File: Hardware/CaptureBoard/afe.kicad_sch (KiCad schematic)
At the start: 64 parts, among them J801 Conn_02x05_Odd_Even, U800 AD9978, U801 ICE40HX4K-BG121, U802 W25Q32JVZP, U803 ADA4800, U804 ADA4800, X801 33.33MHz

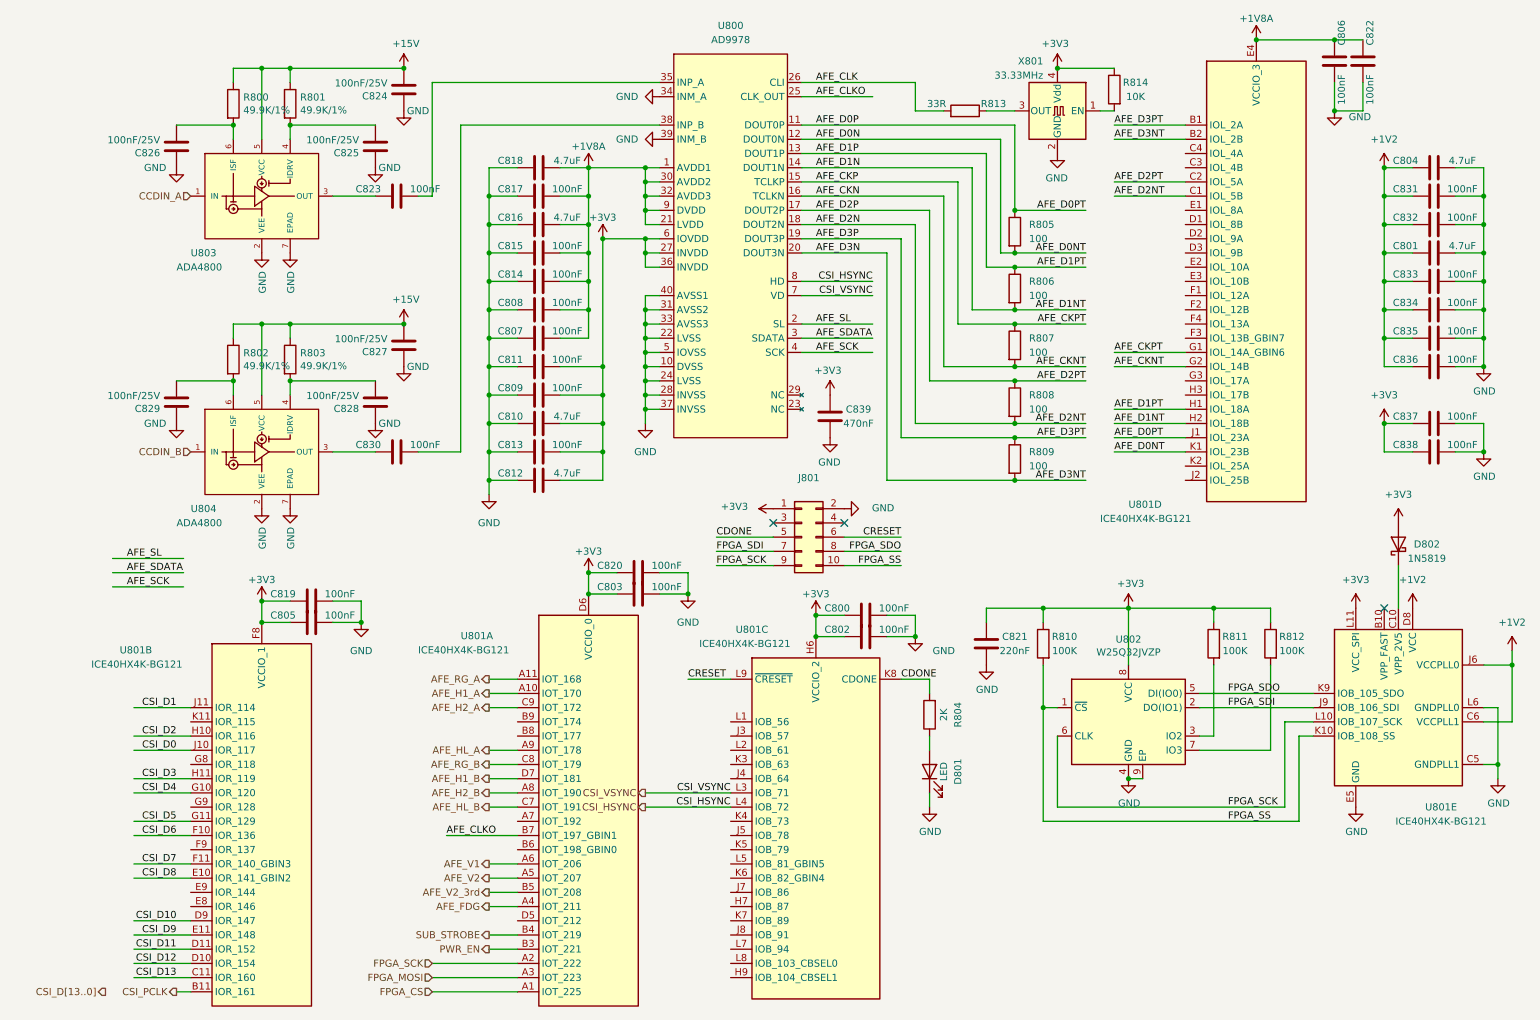
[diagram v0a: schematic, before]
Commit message: pcb: PB r0p2 and CB r0p3 freeze
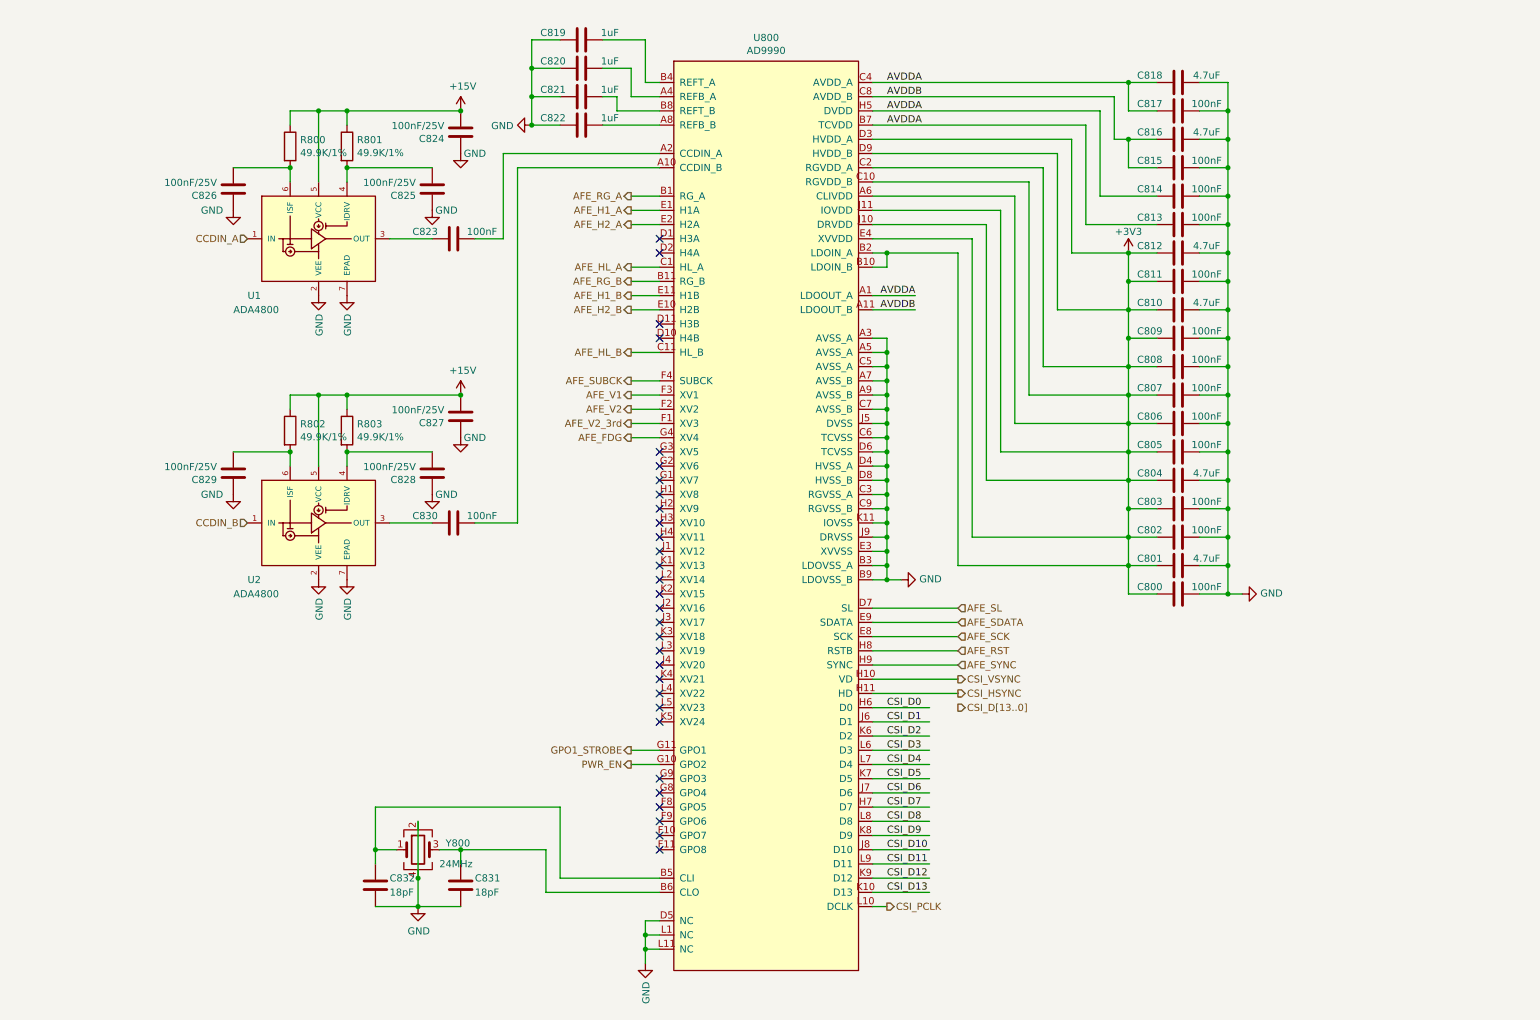
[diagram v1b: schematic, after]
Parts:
- removed C833, C834, C835, C836, C837, C838: 100nF, Capacitor_SMD:C_0402_1005Metric, symbol Device:C
- removed C839: 470nF, Capacitor_SMD:C_0402_1005Metric, symbol Device:C
- removed D801: LED, Diode_SMD:D_0603_1608Metric, symbol Device:LED
- removed D802: 1N5819, Diode_SMD:D_SOD-123, symbol Diode:MBR0530
- removed J801: Conn_02x05_Odd_Even, Connector_PinHeader_1.27mm:PinHeader_2x05_P1.27mm_Vertical_SMD, symbol Connector_Generic:Conn_02x05_Odd_Even
- removed R804: 2K, Resistor_SMD:R_0402_1005Metric, symbol Device:R
- removed R805, R806, R807, R808, R809: 100, Resistor_SMD:R_0402_1005Metric, symbol Device:R
- removed R810, R811, R812: 100K, Resistor_SMD:R_0402_1005Metric, symbol Device:R
- removed R813: 33R, Capacitor_SMD:C_0402_1005Metric, symbol Device:R
- removed R814: 10K, Capacitor_SMD:C_0402_1005Metric, symbol Device:R
- removed U800: AD9978, Package_DFN_QFN:QFN-40-1EP_6x6mm_P0.5mm_EP4.6x4.6mm, symbol Sitina:AD9978
- removed U801: ICE40HX4K-BG121, Package_BGA:BGA-121_9.0x9.0mm_Layout11x11_P0.8mm_Ball0.4mm_Pad0.35mm_NSMD, symbol FPGA_Lattice:ICE40HX4K-BG121
- removed U802: W25Q32JVZP, Package_SON:WSON-8-1EP_6x5mm_P1.27mm_EP3.4x4.3mm, symbol Memory_Flash:W25Q32JVZP
- removed X801: 33.33MHz, Oscillator:Oscillator_SMD_Abracon_ASE-4Pin_3.2x2.5mm, symbol Oscillator:ASE-xxxMHz
- added U800: AD9990, Footprints:BGA-112_11x11_8.0x8.0mm, symbol Sitina:AD9990
- added Y800: 24MHz, Crystal:Crystal_SMD_3225-4Pin_3.2x2.5mm, symbol Device:Crystal_GND24
- C819, C820, C822: value 100nF -> 1uF
- C821: value 220nF -> 1uF
- C831, C832: value 100nF -> 18pF; footprint Capacitor_SMD:C_0402_1005Metric -> Capacitor_SMD:C_0603_1608Metric
- U1: renamed from U803; footprint Package_DFN_QFN:DFN-6-1EP_2x2mm_P0.5mm_EP0.6x1.37mm -> Package_DFN_QFN:DFN-6-1EP_2x1.8mm_P0.5mm_EP1.2x1.6mm
- U2: renamed from U804; footprint Package_DFN_QFN:DFN-6-1EP_2x2mm_P0.5mm_EP0.6x1.37mm -> Package_DFN_QFN:DFN-6-1EP_2x1.8mm_P0.5mm_EP1.2x1.6mm
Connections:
- net +3V3: now also C801.2, C804.2, C806.2, C807.2, C808.2, C809.2, C810.2, C811.2, C812.2, U800.A6 (CLIVDD), U800.B10 (LDOIN_B), U800.B2 (LDOIN_A), U800.C10 (RGVDD_B), U800.C2 (RGVDD_A), U800.D3 (HVDD_A), U800.D9 (HVDD_B), U800.E4 (XVVDD), U800.J10 (DRVDD), U800.J11 (IOVDD); no longer C809.1, C810.1, C811.1, C812.1, C813.1, C819.2, C820.2, C821.2
- net AFE_FDG: now also U800.G4 (XV4)
- net AFE_H1_A: now also U800.E1 (H1A)
- net AFE_H1_B: now also U800.E11 (H1B)
- net AFE_H2_A: now also U800.E2 (H2A)
- net AFE_H2_B: now also U800.E10 (H2B)
- net AFE_HL_A: now also U800.C1 (HL_A)
- net AFE_HL_B: now also U800.C11 (HL_B)
- net AFE_RG_A: now also U800.B1 (RG_A)
- net AFE_RG_B: now also U800.B11 (RG_B)
- net AFE_SCK: now also U800.E8 (SCK)
- net AFE_SDATA: now also U800.E9 (SDATA)
- net AFE_SL: now also U800.D7 (SL)
- net AFE_V1: now also U800.F3 (XV1)
- net AFE_V2: now also U800.F2 (XV2)
- net AFE_V2_3rd: now also U800.F1 (XV3)
- net CSI_D0: now also U800.H6 (D0)
- net CSI_D1: now also U800.J6 (D1)
- net CSI_D10: now also U800.J8 (D10)
- net CSI_D11: now also U800.L9 (D11)
- net CSI_D12: now also U800.K9 (D12)
- net CSI_D13: now also U800.K10 (D13)
- net CSI_D2: now also U800.K6 (D2)
- net CSI_D3: now also U800.L6 (D3)
- net CSI_D4: now also U800.L7 (D4)
- net CSI_D5: now also U800.K7 (D5)
- net CSI_D6: now also U800.J7 (D6)
- net CSI_D7: now also U800.H7 (D7)
- net CSI_D8: now also U800.L8 (D8)
- net CSI_D9: now also U800.K8 (D9)
- net CSI_HSYNC: now also U800.H11 (HD)
- net CSI_PCLK: now also U800.L10 (DCLK)
- net CSI_VSYNC: now also U800.H10 (VD)
- net GND: now also C807.1, C808.1, C809.1, C810.1, C811.1, C812.1, C813.1, C814.1, C815.1, C816.1, C817.1, C818.1, C819.2, C820.2, C821.2, C822.2, U800.A3 (AVSS_A), U800.A5 (AVSS_A), U800.A7 (AVSS_B), U800.A9 (AVSS_B), U800.B3 (LDOVSS_A), U800.B9 (LDOVSS_B), U800.C3 (RGVSS_A), U800.C5 (AVSS_A), U800.C6 (TCVSS), U800.C7 (AVSS_B), U800.C9 (RGVSS_B), U800.D4 (HVSS_A), U800.D5 (NC), U800.D6 (TCVSS), U800.D8 (HVSS_B), U800.E3 (XVVSS), U800.J5 (DVSS), U800.J9 (DRVSS), U800.K11 (IOVSS), U800.L1 (NC), U800.L11 (NC), Y800.2, Y800.4; no longer C807.2, C808.2, C809.2, C810.2, C811.2, C812.2, C813.2, C814.2, C815.2, C816.2, C817.2, C818.2, C819.1, C820.1, C821.1, C822.1
- net PWR_EN: now also U800.G10 (GPO2)
- net at C823.1: now also U800.A2 (CCDIN_A)
- net at C830.1: now also U800.A10 (CCDIN_B)
- removed net +1V2: C801.2, C804.2, C831.2, C832.2
- removed net +1V8A: C806.2, C807.1, C808.1, C814.1, C815.1, C816.1, C817.1, C818.1, C822.2
- new net: C820.1, U800.A4 (REFB_A)
- new net: C822.1, U800.A8 (REFB_B)
- new net: C819.1, U800.B4 (REFT_A)
- new net: C832.2, U800.B5 (CLI), Y800.1
- new net: C831.2, U800.B6 (CLO), Y800.3
- new net: C821.1, U800.B8 (REFT_B)
- new net AFE_RST: U800.H8 (RSTB)
- new net AFE_SUBCK: U800.F4 (SUBCK)
- new net AFE_SYNC: U800.H9 (SYNC)
- new net AVDDA: C813.2, C814.2, C817.2, C818.2, U800.A1 (LDOOUT_A), U800.B7 (TCVDD), U800.C4 (AVDD_A), U800.H5 (DVDD)
- new net AVDDB: C815.2, C816.2, U800.A11 (LDOOUT_B), U800.C8 (AVDD_B)
- new net GPO1_STROBE: U800.G11 (GPO1)
- no-connect marks 3 -> 30
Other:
- moved on the sheet: C800, C801, C802, C803, C804, C805, C806, C807, C808, C809, C810, C811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
